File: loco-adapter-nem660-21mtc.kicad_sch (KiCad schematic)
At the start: 9 parts, among them J701 Conn_02x11_Odd_Even

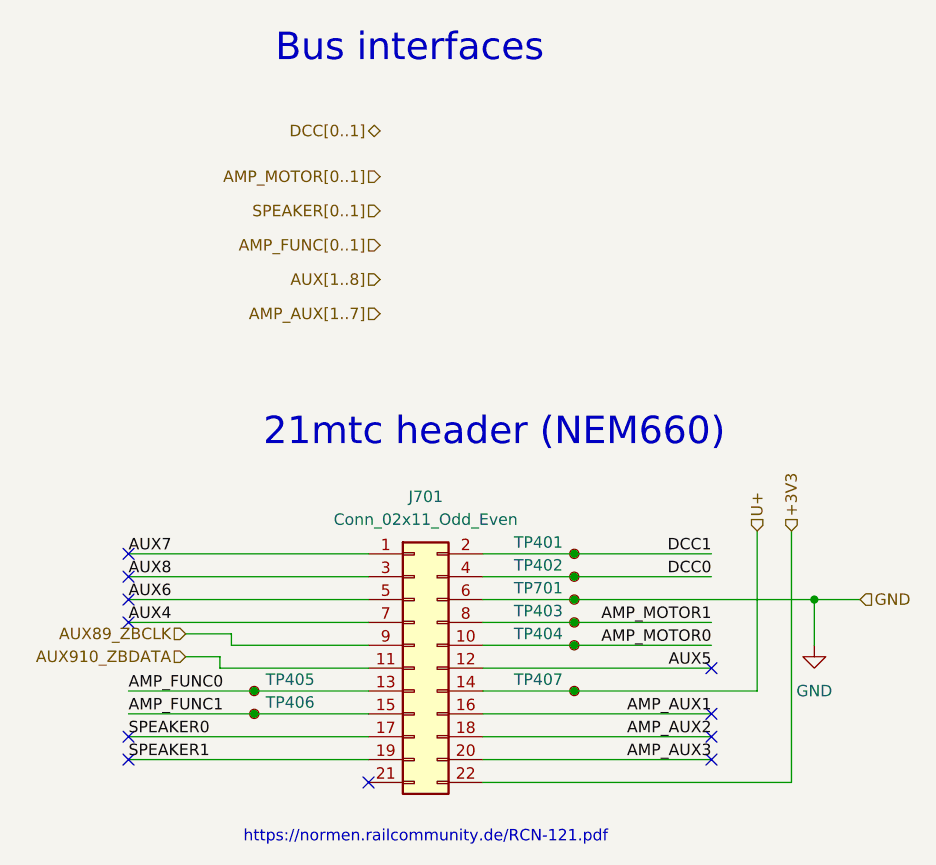
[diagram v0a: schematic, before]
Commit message: Chg - Draft of Plux16 connector
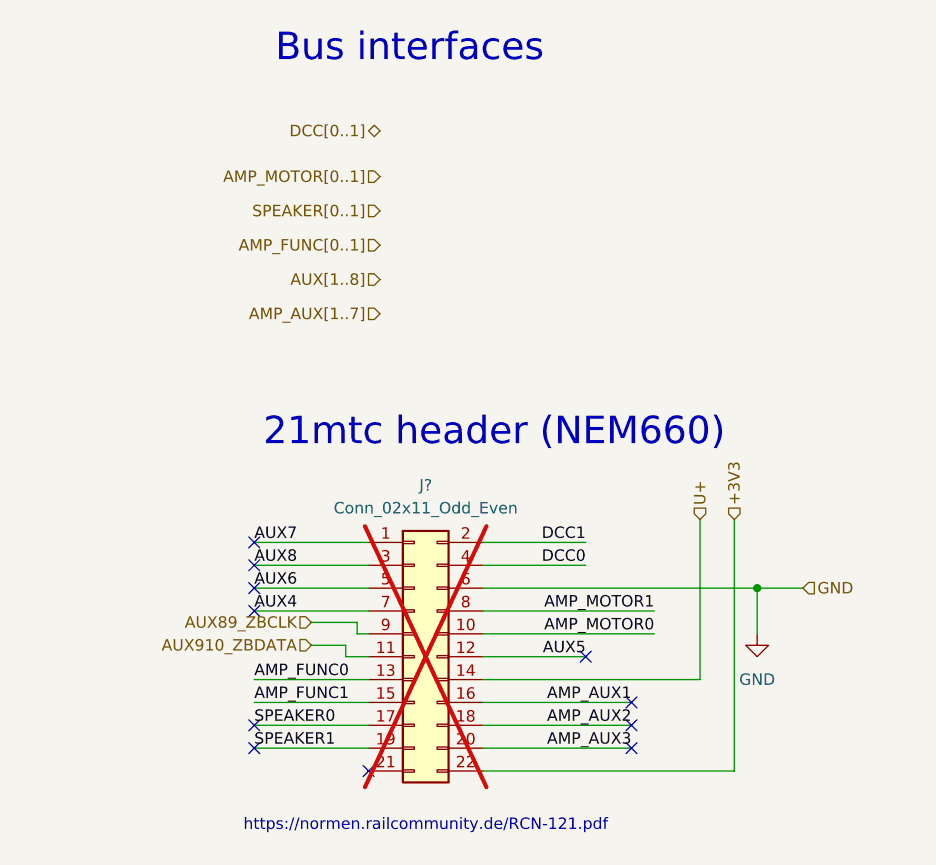
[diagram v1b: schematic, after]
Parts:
- removed TP401, TP402, TP403, TP404, TP405, TP406, TP407, TP701: ~, TestPoint:TestPoint_Pad_D1.0mm, symbol Connector:TestPoint_Small
- J?: renamed from J701; OLI_ID MTC21_02x11_1.27 -> (none); now not fitted; now left out of the parts list
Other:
- company: Chatelain Engineering, Bern - CH -> (none)
- title: xDuinoRail - RailcomDecoder - Development Kit "Hermes" -> (none)
